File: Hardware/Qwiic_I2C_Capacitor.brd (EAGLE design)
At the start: 21.6 x 7.6 mm, 38 parts, among them J1 CONN_02_0603, J2 QWIIC_RIGHT_ANGLE, J3 PTH, U1 NCD2400MDFN

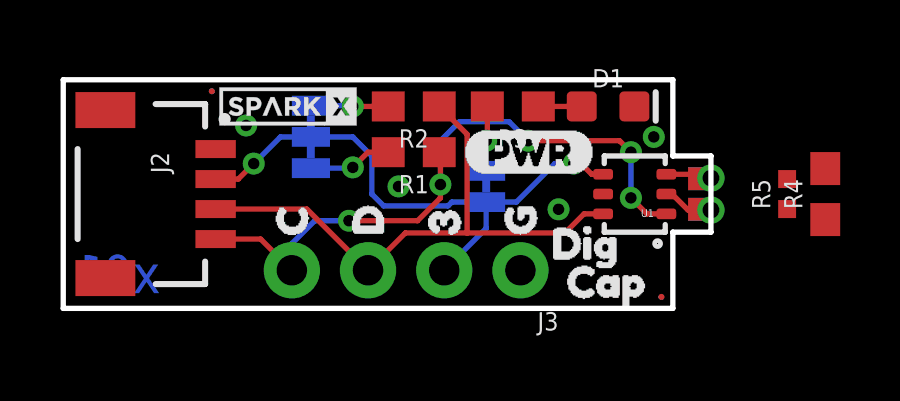
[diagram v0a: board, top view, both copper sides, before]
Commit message: Panelizer/cam output
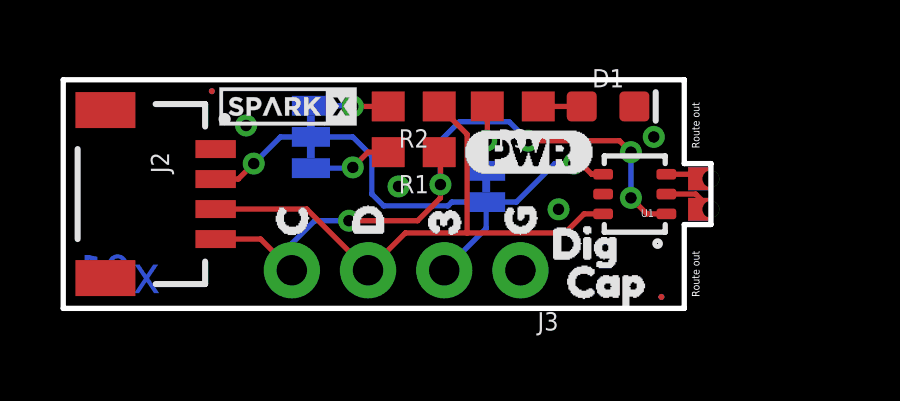
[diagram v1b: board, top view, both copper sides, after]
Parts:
- removed R4: 1k, SparkFun-Resistors:0603
- removed R5: 10k, SparkFun-Resistors:0402-TIGHT
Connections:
- net CN: now also J1.2; no longer J1.P$2
- net CP: now also J1.1; no longer J1.P$1
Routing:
- added copper zone on layer 1, net GND
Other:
- outline, holes or cut-outs redrawn
- board text added: "Route out"
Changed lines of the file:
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@@
 <layer number="27" name="tValues" color="7" fill="1" visible="no" active="yes"/>
 <layer number="28" name="bValues" color="7" fill="1" visible="no" active="yes"/>
-<layer number="29" name="tStop" color="7" fill="3" visible="no" active="yes"/>
-<layer number="30" name="bStop" color="7" fill="6" visible="no" active="yes"/>
+<layer number="29" name="tStop" color="7" fill="3" visible="yes" active="yes"/>
+<layer number="30" name="bStop" color="7" fill="6" visible="yes" active="yes"/>
 <layer number="31" name="tCream" color="7" fill="4" visible="no" active="yes"/>
 <layer number="32" name="bCream" color="7" fill="5" visible="no" active="yes"/>
@@
 <text x="12.7" y="35.56" size="1.778" layer="47" font="vector" ratio="15" align="center">Dimensions in inches</text>
 <text x="35.56" y="39.37" size="1.778" layer="51" font="vector" ratio="15">0.8mm board</text>
-<wire x1="0" y1="0" x2="20.32" y2="0" width="0.1778" layer="20"/>
-<wire x1="20.32" y1="0" x2="20.32" y2="2.54" width="0.1778" layer="20"/>
-<wire x1="20.32" y1="2.54" x2="21.59" y2="2.54" width="0.1778" layer="20"/>
-<wire x1="21.59" y1="2.54" x2="21.59" y2="5.08" width="0.1778" layer="20"/>
-<wire x1="21.59" y1="5.08" x2="20.32" y2="5.08" width="0.1778" layer="20"/>
-<wire x1="20.32" y1="5.08" x2="20.32" y2="7.62" width="0.1778" layer="20"/>
-<wire x1="20.32" y1="7.62" x2="0" y2="7.62" width="0.1778" layer="20"/>
+<wire x1="0" y1="0" x2="20.701" y2="0" width="0.1778" layer="20"/>
+<wire x1="20.701" y1="0" x2="20.701" y2="2.794" width="0.1778" layer="20"/>
+<wire x1="20.701" y1="2.794" x2="21.59" y2="2.794" width="0.1778" layer="20"/>
+<wire x1="21.59" y1="2.794" x2="21.59" y2="4.826" width="0.1778" layer="20"/>
+<wire x1="21.59" y1="4.826" x2="20.701" y2="4.826" width="0.1778" layer="20"/>
+<wire x1="20.701" y1="4.826" x2="20.701" y2="7.62" width="0.1778" layer="20"/>
+<wire x1="20.701" y1="7.62" x2="0" y2="7.62" width="0.1778" layer="20"/>
 <wire x1="0" y1="7.62" x2="0" y2="0" width="0.1778" layer="20"/>
-<rectangle x1="20.828" y1="3.937" x2="21.59" y2="4.699" layer="1"/>
-<rectangle x1="20.828" y1="2.921" x2="21.59" y2="3.683" layer="1"/>
-<rectangle x1="20.828" y1="3.937" x2="21.59" y2="4.699" layer="16"/>
-<rectangle x1="20.828" y1="2.921" x2="21.59" y2="3.683" layer="16"/>
-<rectangle x1="20.828" y1="3.937" x2="21.59" y2="4.699" layer="29"/>
-<rectangle x1="20.828" y1="2.921" x2="21.59" y2="3.683" layer="29"/>
-<rectangle x1="20.828" y1="3.937" x2="21.59" y2="4.699" layer="30"/>
-<rectangle x1="20.828" y1="2.921" x2="21.59" y2="3.683" layer="30"/>
-<rectangle x1="21.59" y1="2.54" x2="22.86" y2="3.81" layer="30"/>
 <text x="19.05" y="-11.43" size="1.778" layer="51" font="vector" ratio="15">Priyanka Makin</text>
+<text x="21.209" y="5.334" size="0.254" layer="20" font="vector" ratio="15" rot="R90">Route out</text>
+<text x="21.209" y="0.381" size="0.254" layer="20" font="vector" ratio="15" rot="R90">Route out</text>
 </plain>
 <attributes>
@@
 </class>
 </classes>
-<designrules name="SparkFun-2-layer-TIGHT">
+<designrules name="SparkFun-2-layer-TIGHT *">
 <description language="en">&lt;b&gt;SparkFun 2 Layer Design Rule Checks - STANDARD/TIGHT/FAB-LIMIT&lt;/b&gt;
 &lt;p&gt;
@@
 <param name="msMicroVia" value="9.99mm"/>
 <param name="msBlindViaRatio" value="0.5"/>
-<param name="rvPadTop" value="0.25"/>
-<param name="rvPadInner" value="0.25"/>
-<param name="rvPadBottom" value="0.25"/>
+<param name="rvPadTop" value="0"/>
+<param name="rvPadInner" value="0"/>
+<param name="rvPadBottom" value="0"/>
 <param name="rvViaOuter" value="0.25"/>
 <param name="rvViaInner" value="0.25"/>
 <param name="rvMicroViaOuter" value="0.25"/>
 <param name="rvMicroViaInner" value="0.25"/>
-<param name="rlMinPadTop" value="7mil"/>
+<param name="rlMinPadTop" value="0mil"/>
 <param name="rlMaxPadTop" value="20mil"/>
 <param name="rlMinPadInner" value="7mil"/>
 <param name="rlMaxPadInner" value="20mil"/>
-<param name="rlMinPadBottom" value="7mil"/>
+<param name="rlMinPadBottom" value="0mil"/>
 <param name="rlMaxPadBottom" value="20mil"/>
 <param name="rlMinViaOuter" value="7mil"/>
@@
 <element name="U$20" library="Labels" package="QWIIC_COPYRIGHT_SMALL" value="" x="1.27" y="3.81" smashed="yes" rot="MR90"/>
 <element name="U$21" library="Labels" package="QWIIC_COPYRIGHT_SMALL" value="" x="1.27" y="3.81" smashed="yes" rot="MR90"/>
-<element name="R4" library="SparkFun-Resistors" package="0603" value="1k" x="25.4" y="3.81" smashed="yes" rot="R90">
-<attribute name="NAME" x="24.638" y="3.81" size="0.6096" layer="25" font="vector" ratio="20" rot="R90" align="bottom-center"/>
-<attribute name="PROD_ID" value="RES-07856" x="25.4" y="3.81" size="1.778" layer="27" font="vector" ratio="15" rot="R90" display="off"/>
-<attribute name="VALUE" x="26.162" y="3.81" size="0.6096" layer="27" font="vector" ratio="20" rot="R90" align="top-center"/>
-</element>
-<element name="R5" library="SparkFun-Resistors" package="0402-TIGHT" value="10k" x="24.13" y="3.81" smashed="yes" rot="R90">
-<attribute name="NAME" x="23.568" y="3.81" size="0.6096" layer="25" font="vector" ratio="20" rot="R90" align="bottom-center"/>
-<attribute name="PROD_ID" value="RES-14241" x="24.13" y="3.81" size="1.778" layer="27" font="vector" ratio="15" rot="R90" display="off"/>
-<attribute name="VALUE" x="24.692" y="3.81" size="0.6096" layer="27" font="vector" ratio="20" rot="R90" align="top-center"/>
-</element>
 <element name="LOGO2" library="SparkFun-Aesthetics" package="ORDERING_INSTRUCTIONS" value="SPECIAL_INSTRUCTIONS-ORDERING" x="31.75" y="53.34" smashed="yes"/>
 <element name="J1" library="Qwiic_Capacitor" package="0603_CASTELLATED" value="CONN_02_0603" x="21.59" y="3.81" smashed="yes" rot="R90"/>
@@
 <polygon width="0.1778" layer="16" isolate="0.3048">
 <vertex x="0" y="0"/>
-<vertex x="20.32" y="0"/>
-<vertex x="20.32" y="2.54"/>
-<vertex x="21.59" y="2.54"/>
-<vertex x="21.59" y="5.08"/>
-<vertex x="20.32" y="5.08"/>
-<vertex x="20.32" y="7.62"/>
+<vertex x="20.701" y="0"/>
+<vertex x="20.701" y="2.794"/>
+<vertex x="21.59" y="2.794"/>
+<vertex x="21.59" y="4.826"/>
+<vertex x="20.701" y="4.826"/>
+<vertex x="20.701" y="7.62"/>
 <vertex x="0" y="7.62"/>
 </polygon>
-<polygon width="0.1778" layer="16" isolate="0.3048">
+<polygon width="0.1778" layer="1" isolate="0.3048">
 <vertex x="0" y="0"/>
-<vertex x="20.32" y="0"/>
-<vertex x="20.32" y="2.54"/>
-<vertex x="21.59" y="2.54"/>
-<vertex x="21.59" y="5.08"/>
-<vertex x="20.32" y="5.08"/>
-<vertex x="20.32" y="7.62"/>
+<vertex x="20.701" y="0"/>
+<vertex x="20.701" y="2.794"/>
+<vertex x="21.59" y="2.794"/>
+<vertex x="21.59" y="4.826"/>
+<vertex x="20.701" y="4.826"/>
+<vertex x="20.701" y="7.62"/>
 <vertex x="0" y="7.62"/>
 </polygon>
@@
 <signal name="CP">
 <contactref element="U1" pad="2"/>
-<contactref element="J1" pad="P$1"/>
-<wire x1="21.59" y1="3.2766" x2="20.828" y2="3.2766" width="0.1778" layer="1"/>
-<wire x1="20.828" y1="3.2766" x2="20.2946" y2="3.81" width="0.1778" layer="1"/>
-<wire x1="20.2946" y1="3.81" x2="20.1041" y2="3.81" width="0.1778" layer="1"/>
+<contactref element="J1" pad="1"/>
+<wire x1="21.59" y1="3.302" x2="21.082" y2="3.81" width="0.1778" layer="1"/>
+<wire x1="21.082" y1="3.81" x2="20.1041" y2="3.81" width="0.1778" layer="1"/>
 </signal>
 <signal name="CN">
 <contactref element="U1" pad="3"/>
-<contactref element="J1" pad="P$2"/>
-<wire x1="21.59" y1="4.3434" x2="21.463" y2="4.4704" width="0.1778" layer="1"/>
-<wire x1="21.463" y1="4.4704" x2="20.1041" y2="4.4704" width="0.1778" layer="1"/>
+<contactref element="J1" pad="2"/>
+<wire x1="21.59" y1="4.318" x2="21.4376" y2="4.4704" width="0.1778" layer="1"/>
+<wire x1="21.4376" y1="4.4704" x2="20.1041" y2="4.4704" width="0.1778" layer="1"/>
 </signal>
 </signals>
